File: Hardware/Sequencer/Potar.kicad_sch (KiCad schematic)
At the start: 17 parts, among them U501 MCP23017_SP

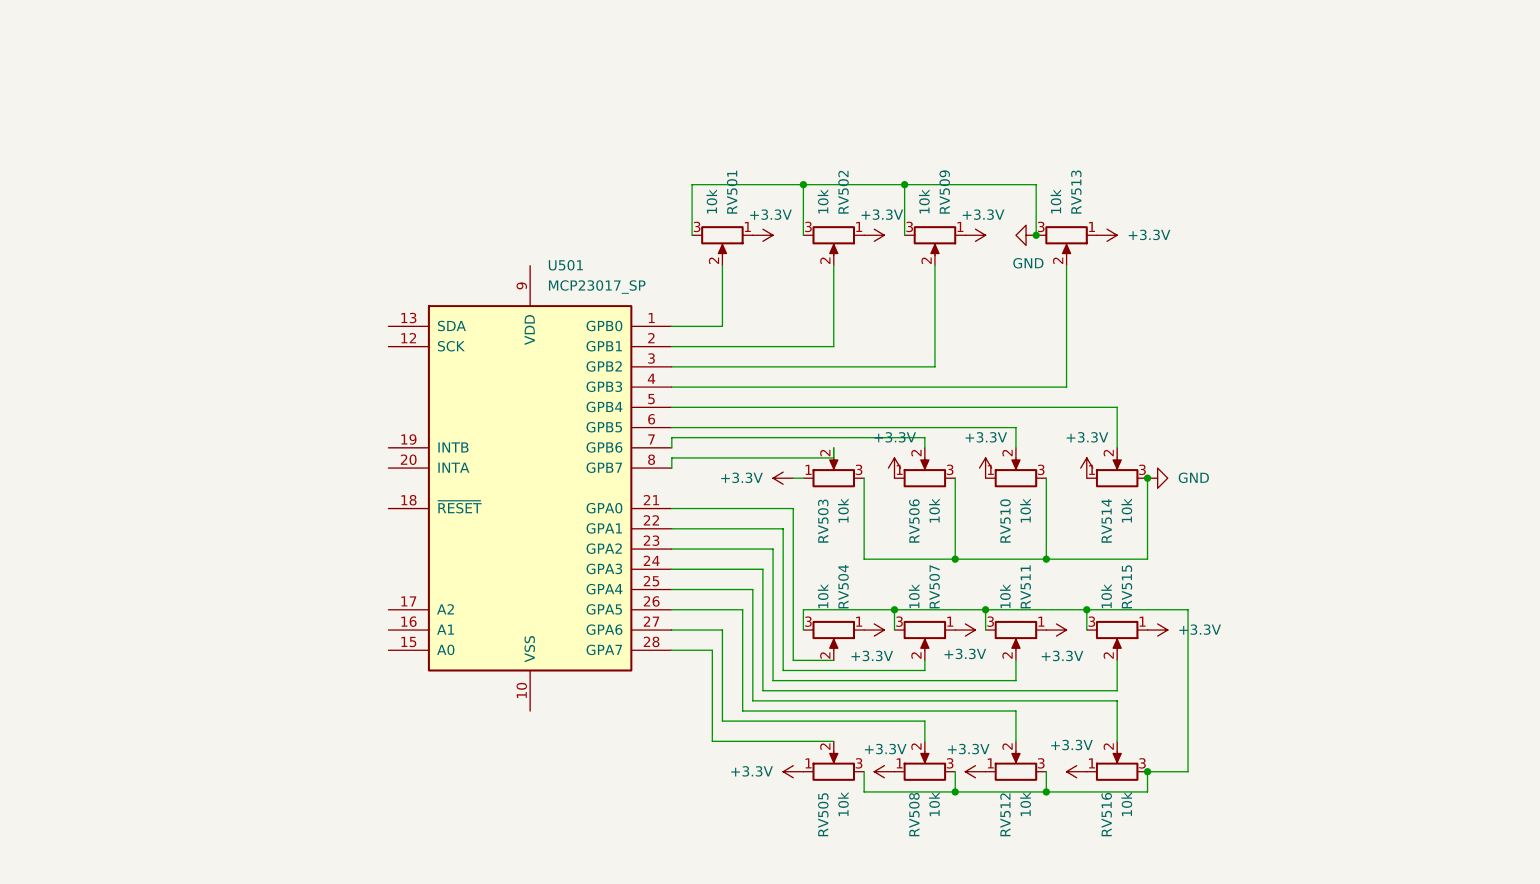
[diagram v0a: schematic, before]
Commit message: project add
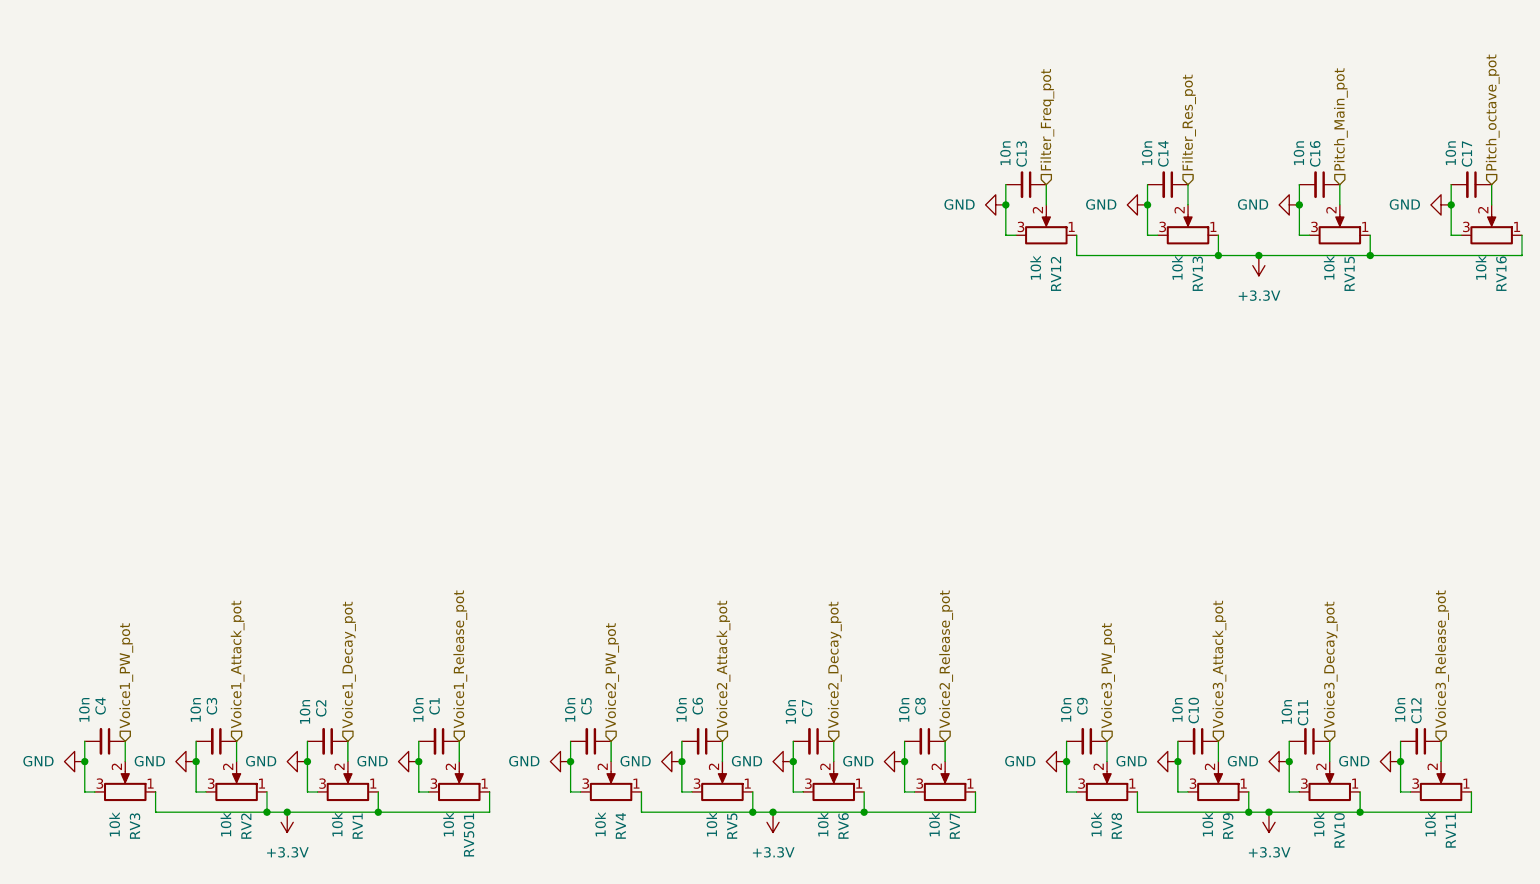
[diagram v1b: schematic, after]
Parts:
- removed RV502, RV503, RV504, RV505, RV506, RV507, RV508, RV509, RV510, RV511, RV512, RV513, RV514, RV515, RV516: 10k, symbol Device:R_Potentiometer
- removed U501: MCP23017_SP, Package_DIP:DIP-28_W7.62mm, symbol Interface_Expansion:MCP23017_SP
- added C1, C10, C11, C12, C13, C14, C16, C17, C2, C3, C4, C5, C6, C7, C8, C9: 10n, symbol Device:C_Small
- added RV1, RV10, RV11, RV12, RV13, RV15, RV16, RV2, RV3, RV4, RV5, RV6, RV7, RV8, RV9: 10k, symbol Device:R_Potentiometer
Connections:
- net +3.3V: now also RV1.1, RV10.1, RV11.1, RV12.1, RV13.1, RV15.1, RV16.1, RV2.1, RV3.1, RV4.1, RV5.1, RV6.1, RV7.1, RV8.1, RV9.1
- net GND: now also C1.2, C10.2, C11.2, C12.2, C13.2, C14.2, C16.2, C17.2, C2.2, C3.2, C4.2, C5.2, C6.2, C7.2, C8.2, C9.2, RV1.3, RV10.3, RV11.3, RV12.3, RV13.3, RV15.3, RV16.3, RV2.3, RV3.3, RV4.3, RV5.3, RV6.3, RV7.3, RV8.3, RV9.3
- net Voice1_Release_pot: now reaches RV501.2
- net Voice1_Release_pot: now also C1.1
- new net Filter_Freq_pot: C13.1, RV12.2
- new net Filter_Res_pot: C14.1, RV13.2
- new net Pitch_Main_pot: C16.1, RV15.2
- new net Pitch_octave_pot: C17.1, RV16.2
- new net Voice1_Attack_pot: C3.1, RV2.2
- new net Voice1_Decay_pot: C2.1, RV1.2
- new net Voice1_PW_pot: C4.1, RV3.2
- new net Voice2_Attack_pot: C6.1, RV5.2
- new net Voice2_Decay_pot: C7.1, RV6.2
- new net Voice2_PW_pot: C5.1, RV4.2
- new net Voice2_Release_pot: C8.1, RV7.2
- new net Voice3_Attack_pot: C10.1, RV9.2
- new net Voice3_Decay_pot: C11.1, RV10.2
- new net Voice3_PW_pot: C9.1, RV8.2
- new net Voice3_Release_pot: C12.1, RV11.2
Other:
- title: (none) -> Potars
- moved on the sheet: RV501
